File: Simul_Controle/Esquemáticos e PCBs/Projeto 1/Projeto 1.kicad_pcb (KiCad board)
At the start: 2 copper layers, 50 x 50 mm, 11 parts, among them J1 Conn_01x03_Pin, J2 Conn_01x02, J3 Conn_01x02, U1 LF355

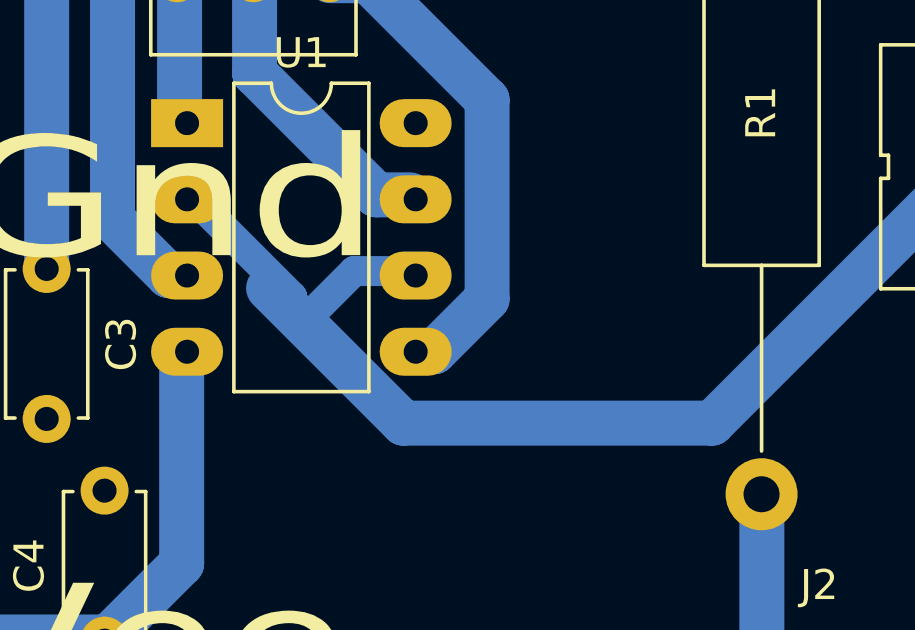
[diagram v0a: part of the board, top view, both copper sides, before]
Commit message: Adicionado conversor flyback
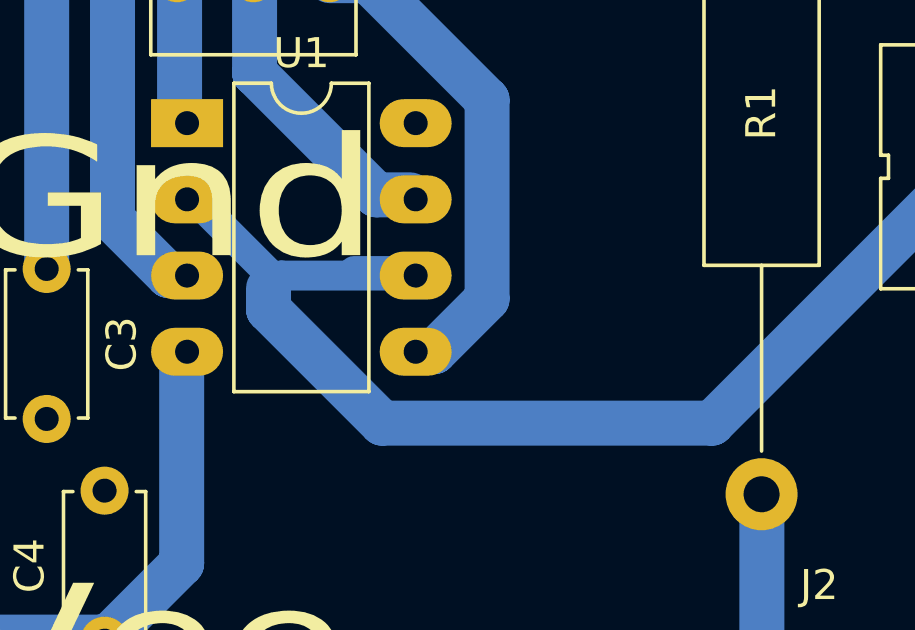
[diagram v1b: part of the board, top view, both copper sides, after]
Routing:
- net Vout: track 52.7 -> 54.9 mm
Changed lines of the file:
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@@
   (segment (start 59.69 37.34) (end 57.76 39.27) (width 1.5) (layer "B.Cu") (net 2))
   (segment (start 66.14 35.18) (end 66.16 35.2) (width 1.5) (layer "B.Cu") (net 2))
-  (segment (start 42.09 58.095837) (end 42.09 58.39) (width 1) (layer "B.Cu") (net 3))
+  (segment (start 41.305 57.310837) (end 41.305 57.822717) (width 1) (layer "B.Cu") (net 3))
   (segment (start 66.54 51.87) (end 66.54 40.58) (width 1.5) (layer "B.Cu") (net 3))
+  (segment (start 46.03 57.25) (end 44.16 57.25) (width 1) (layer "B.Cu") (net 3))
+  (segment (start 41.727717 57.4) (end 41.305 57.822717) (width 1) (layer "B.Cu") (net 3))
+  (segment (start 66.54 40.58) (end 66.16 40.2) (width 1.5) (layer "B.Cu") (net 3))
+  (segment (start 41.305 58.535) (end 41.305 57.822717) (width 1.5) (layer "B.Cu") (net 3))
+  (segment (start 46.21 57.4) (end 41.727717 57.4) (width 1) (layer "B.Cu") (net 3))
+  (segment (start 45.09 62.32) (end 41.305 58.535) (width 1.5) (layer "B.Cu") (net 3))
+  (segment (start 38.854163 54.86) (end 41.305 57.310837) (width 1) (layer "B.Cu") (net 3))
+  (segment (start 56.09 62.32) (end 45.09 62.32) (width 1.5) (layer "B.Cu") (net 3))
+  (segment (start 38.59 54.86) (end 38.854163 54.86) (width 1) (layer "B.Cu") (net 3))
   (segment (start 66.54 51.87) (end 56.09 62.32) (width 1.5) (layer "B.Cu") (net 3))
-  (segment (start 38.59 54.86) (end 38.854163 54.86) (width 1) (layer "B.Cu") (net 3))
-  (segment (start 46.03 57.25) (end 44.16 57.25) (width 1) (layer "B.Cu") (net 3))
-  (segment (start 56.09 62.32) (end 45.802283 62.32) (width 1.5) (layer "B.Cu") (net 3))
-  (segment (start 45.802283 62.32) (end 41.305 57.822717) (width 1.5) (layer "B.Cu") (net 3))
-  (segment (start 66.54 40.58) (end 66.16 40.2) (width 1.5) (layer "B.Cu") (net 3))
-  (segment (start 44.16 57.25) (end 42.446141 58.963859) (width 1) (layer "B.Cu") (net 3))
-  (segment (start 38.854163 54.86) (end 42.09 58.095837) (width 1) (layer "B.Cu") (net 3))
   (segment (start 40.84 50.65137) (end 44.89863 54.71) (width 1.5) (layer "B.Cu") (net 4))
   (segment (start 40.8 47.57) (end 40.84 47.61) (width 1.5) (layer "B.Cu") (net 4))
